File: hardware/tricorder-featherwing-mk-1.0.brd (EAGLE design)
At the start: 50.8 x 25.4 mm, 7 parts, among them U1 ADAFRUIT_FEATHER_SHIELDSMALLH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

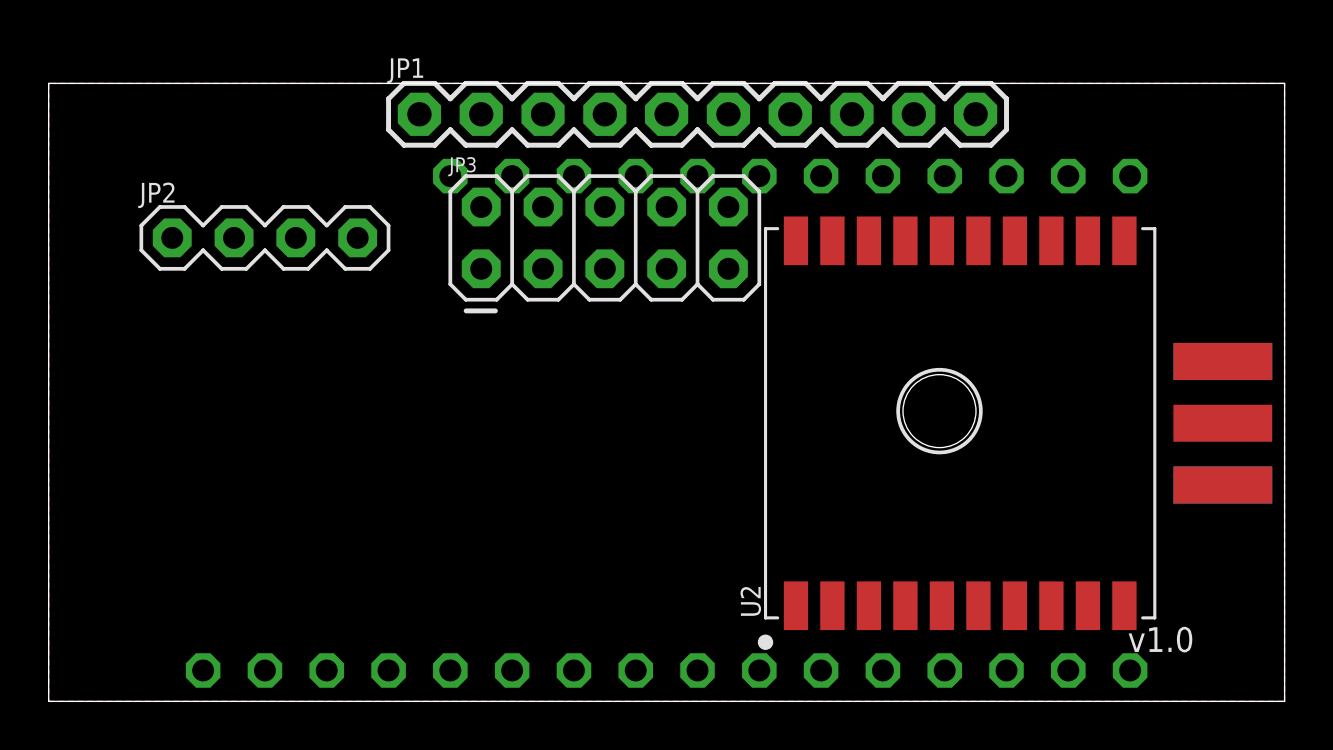
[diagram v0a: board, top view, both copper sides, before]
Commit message: connector board markup?
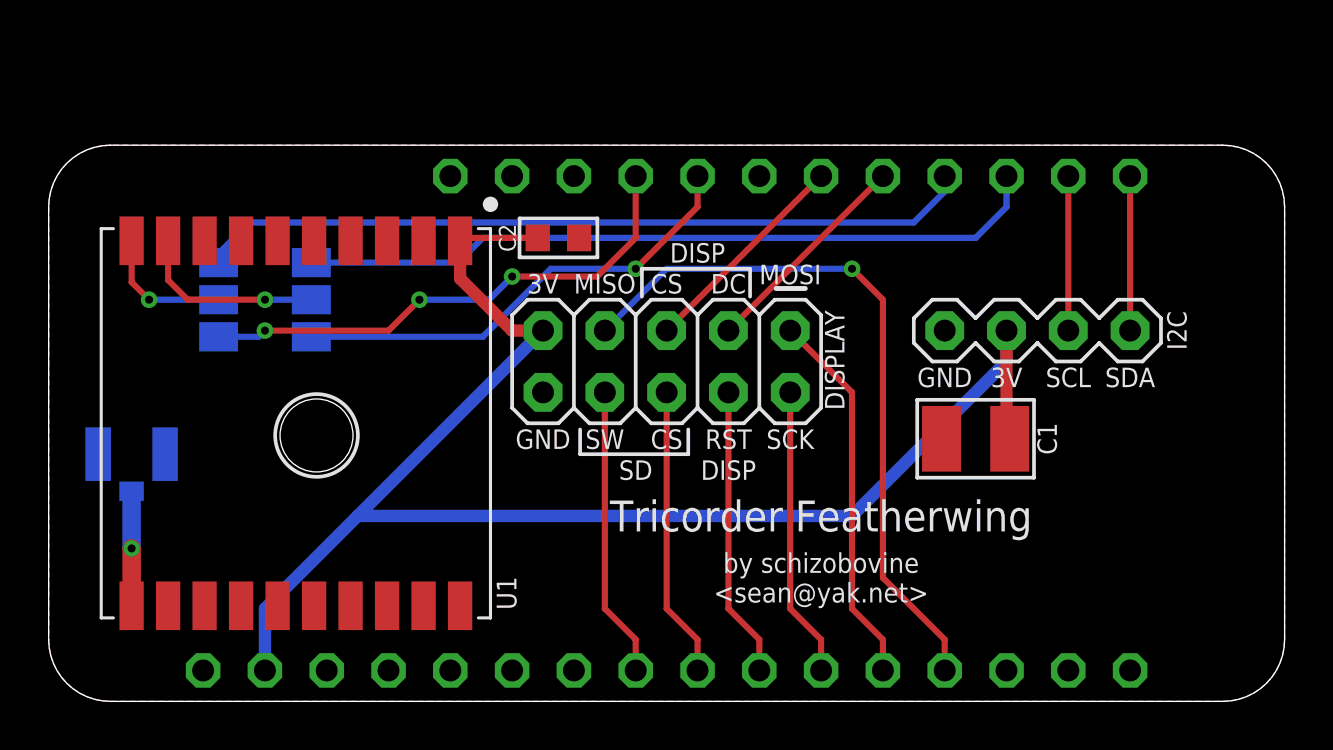
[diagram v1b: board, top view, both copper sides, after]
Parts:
- removed J$1: SMA_EDGE, a_parts:SMA-EDGE
- removed JP1: M10PTH, a_parts:1X10
- removed JP2: M04PTH, a_parts:1X04-PTH-VERT
- removed JP3: M05X2PTH, a_parts:AVR_ICSP
- removed U2: (no value), a_parts:FGPMMOPA6H
- added C1: 10uF, a_parts:C1210
- added C2: 1uF, a_parts:C0603
- added DISPLAY: M05X2PTH, a_parts:AVR_ICSP
- added FEATHERWING: ADAFRUIT_FEATHER_SHIELDSMALLHOLES_NS, a_parts:ADAFRUIT_FEATHER_SMALLHOLES_NS
- added GPS_ANT: (no value), a_parts:U.FL
- added GPS_RX, GPS_TX: (no value), a_parts:PAD-JUMPER-3-NO_YES_SILK_FULL_BOX
- added I2C: M04PTH, a_parts:1X04-PTH-VERT
- U1: value ADAFRUIT_FEATHER_SHIELDSMALLHOLES_NS -> (none); device a_parts:ADAFRUIT_FEATHER_SMALLHOLES_NS -> a_parts:FGPMMOPA6H
- moved U1 15.2 mm to (10.2, 11.4), turned to 270 degrees
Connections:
- new net 3.3V: C1.1, C2.1, DISPLAY.9, FEATHERWING.3V, I2C.2, U1.P$1
- new net DISP_CS: DISPLAY.5, FEATHERWING.10
- new net DISP_DC: DISPLAY.3, FEATHERWING.9
- new net DISP_RST: DISPLAY.4, FEATHERWING.A5
- new net GND: C1.2, C2.2, DISPLAY.10, FEATHERWING.GND@0, FEATHERWING.GND@1, GPS_ANT.1, GPS_ANT.2, I2C.1, U1.P$12, U1.P$19, U1.P$3, U1.P$8
- new net GPS_RX: GPS_RX.2, U1.P$10
- new net GPS_RX1: FEATHERWING.6, GPS_RX.1
- new net GPS_RX2: FEATHERWING.13, GPS_RX.3
- new net GPS_TX: GPS_TX.2, U1.P$9
- new net GPS_TX1: FEATHERWING.5, GPS_TX.3
- new net GPS_TX2: FEATHERWING.12, GPS_TX.1
- new net MISO: DISPLAY.7, FEATHERWING.MISO
- new net MOSI: DISPLAY.1, FEATHERWING.MOSI
- new net SCK: DISPLAY.2, FEATHERWING.SCK
- new net SCL: FEATHERWING.SCL, I2C.3
- new net SDA: FEATHERWING.SDA, I2C.4
- new net SD_CS: DISPLAY.6, FEATHERWING.A4
- new net SD_SW: DISPLAY.8, FEATHERWING.A3
- net N$1: now also GPS_ANT.3, U1.P$11; no longer J$1.SIG, U2.P$11
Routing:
- net 3.3V: track 0.00 -> 62.9 mm
- net GPS_RX1: track 0.00 -> 31.9 mm
- net GPS_TX1: track 0.00 -> 30.8 mm
- net MISO: track 0.00 -> 29.3 mm, vias 0 -> 1
- net GPS_RX2: track 0.00 -> 21.4 mm, vias 0 -> 3
- net GPS_TX2: track 0.00 -> 19.4 mm, vias 0 -> 1
- net MOSI: track 0.00 -> 15.5 mm
- net SD_CS: track 0.00 -> 12.0 mm
- net SD_SW: track 0.00 -> 12.0 mm
- net SCK: track 0.00 -> 12.0 mm
- net DISP_RST: track 0.00 -> 12.0 mm
- net DISP_CS: track 0.00 -> 8.98 mm
- net DISP_DC: track 0.00 -> 8.98 mm
- net GPS_TX: track 0.00 -> 7.83 mm, vias 0 -> 1
- net SDA: track 0.00 -> 6.35 mm
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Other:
- board size 50.8 x 25.4 mm -> 50.8 x 22.9 mm
- board text added: "3V"
- board text added: "CS"
- board text added: "DC"
- board text added: "DISP"
- board text added: "GND"
- board text added: "MISO"
- board text added: "MOSI"
- board text added: "RST"
- board text added: "SCK"
- board text added: "SCL"
- board text added: "SD"
- board text added: "SDA"
- board text added: "SW"
- board text added: "Tricorder Featherwing"
- board text added: "by schizobovine <sean@yak.net>"
